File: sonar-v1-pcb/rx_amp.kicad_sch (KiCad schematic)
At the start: 7 parts, among them U10 ${SIM.PARAMS}, U11 ${SIM.PARAMS}

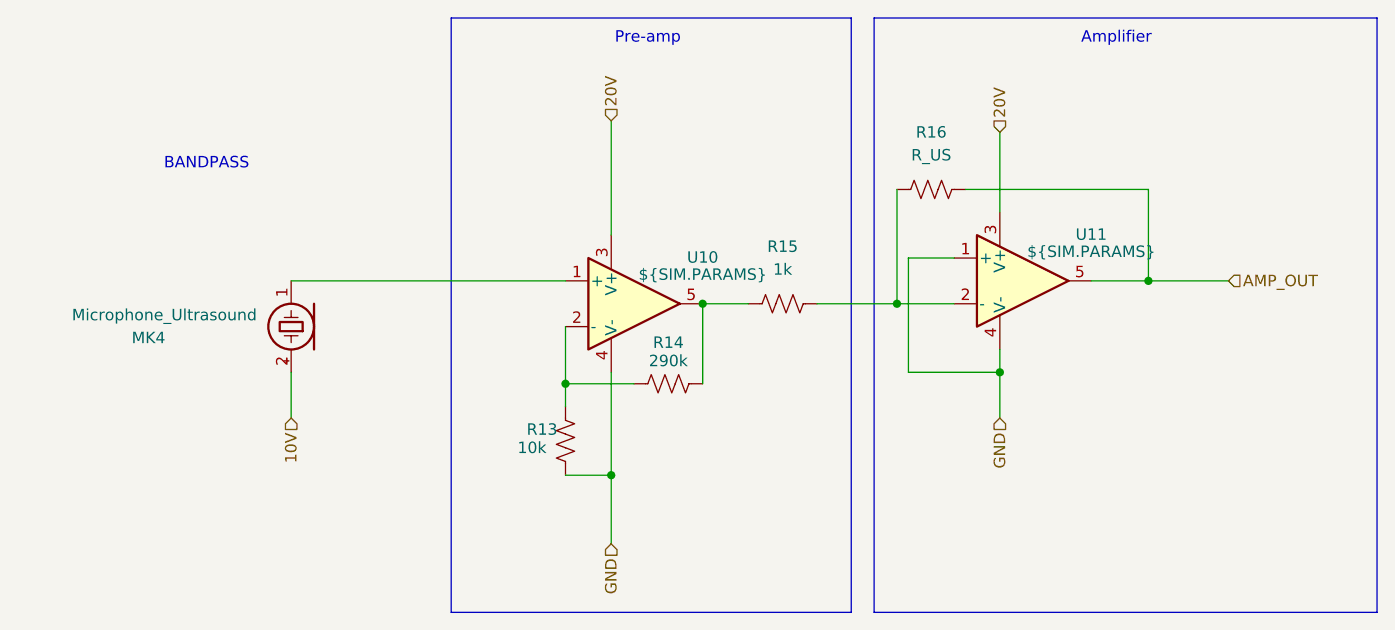
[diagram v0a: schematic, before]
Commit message: added some adc shit
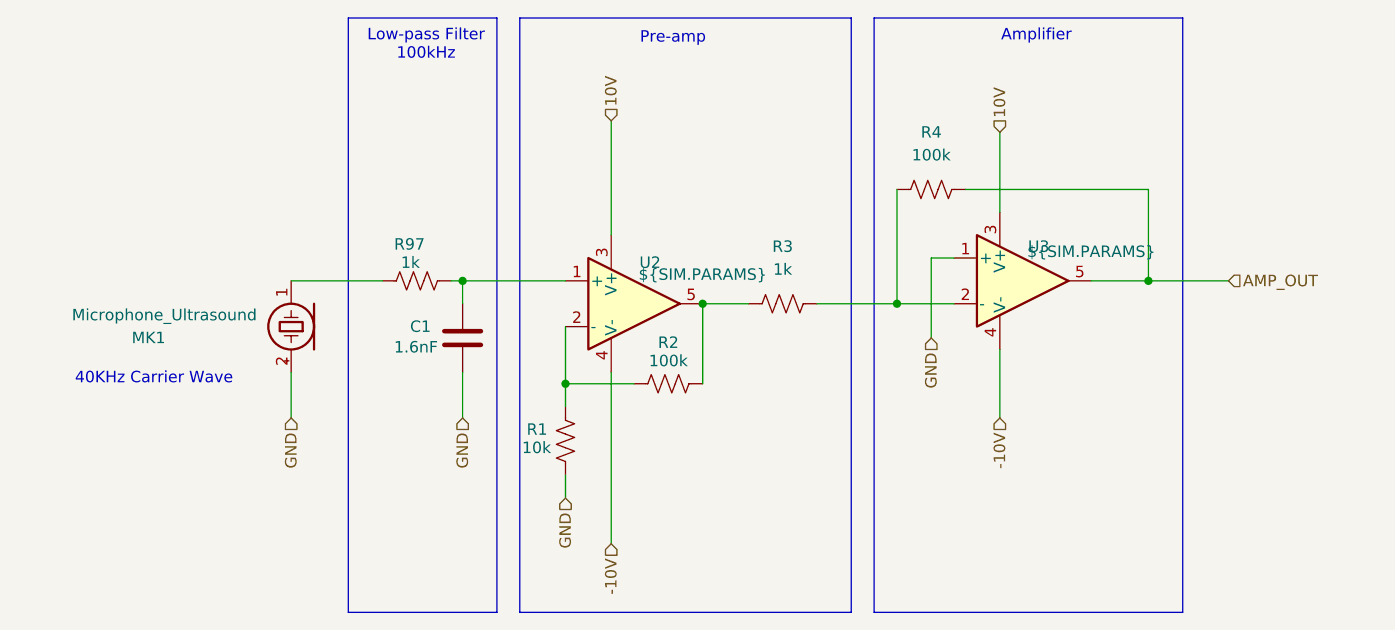
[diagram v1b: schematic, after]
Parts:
- added C1: 1.6nF, Capacitor_SMD:C_0201_0603Metric, symbol Device:C
- added R97: 1k, Resistor_SMD:R_0201_0603Metric, symbol Device:R_US
- R1: renamed from R13; footprint Capacitor_SMD:C_0201_0603Metric -> Resistor_SMD:R_0201_0603Metric
- R2: renamed from R14; value 290k -> 100k; footprint Capacitor_SMD:C_0201_0603Metric -> Resistor_SMD:R_0201_0603Metric
- R3: renamed from R15; footprint Capacitor_SMD:C_0201_0603Metric -> Resistor_SMD:R_0201_0603Metric
- R4: renamed from R16; value R_US -> 100k; footprint (none) -> Resistor_SMD:R_0201_0603Metric
- U2: renamed from U10; footprint (none) -> Package_TO_SOT_SMD:SOT-23-5
- U3: renamed from U11; footprint (none) -> Package_TO_SOT_SMD:SOT-23-5
- renumbered MK4 to MK1
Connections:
- net 20V is gone; now on net 10V: U2.3 (V+), U3.3 (V+)
- net 10V: no longer MK1.2 (+)
- net GND: now also MK1.2 (+), C1.2; no longer U2.4 (V-), U3.4 (V-)
- net at U2.1 (+): now also C1.1, R97.1; no longer MK1.1 (-)
- new net: MK1.1 (-), R97.2
- new net -10V: U2.4 (V-), U3.4 (V-)
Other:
- note added: "40KHz Carrier Wave"
- note added: "Low-pass Filter 100kHz"
- note removed: "BANDPASS"
